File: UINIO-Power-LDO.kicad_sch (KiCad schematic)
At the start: 24 parts, among them J1 Conn_01x03_Pin, U1 ME6211C33M5G-N, U2 XC6206PxxxMR, U3 SGM2019-3.3YN5G, U4 AMS1117

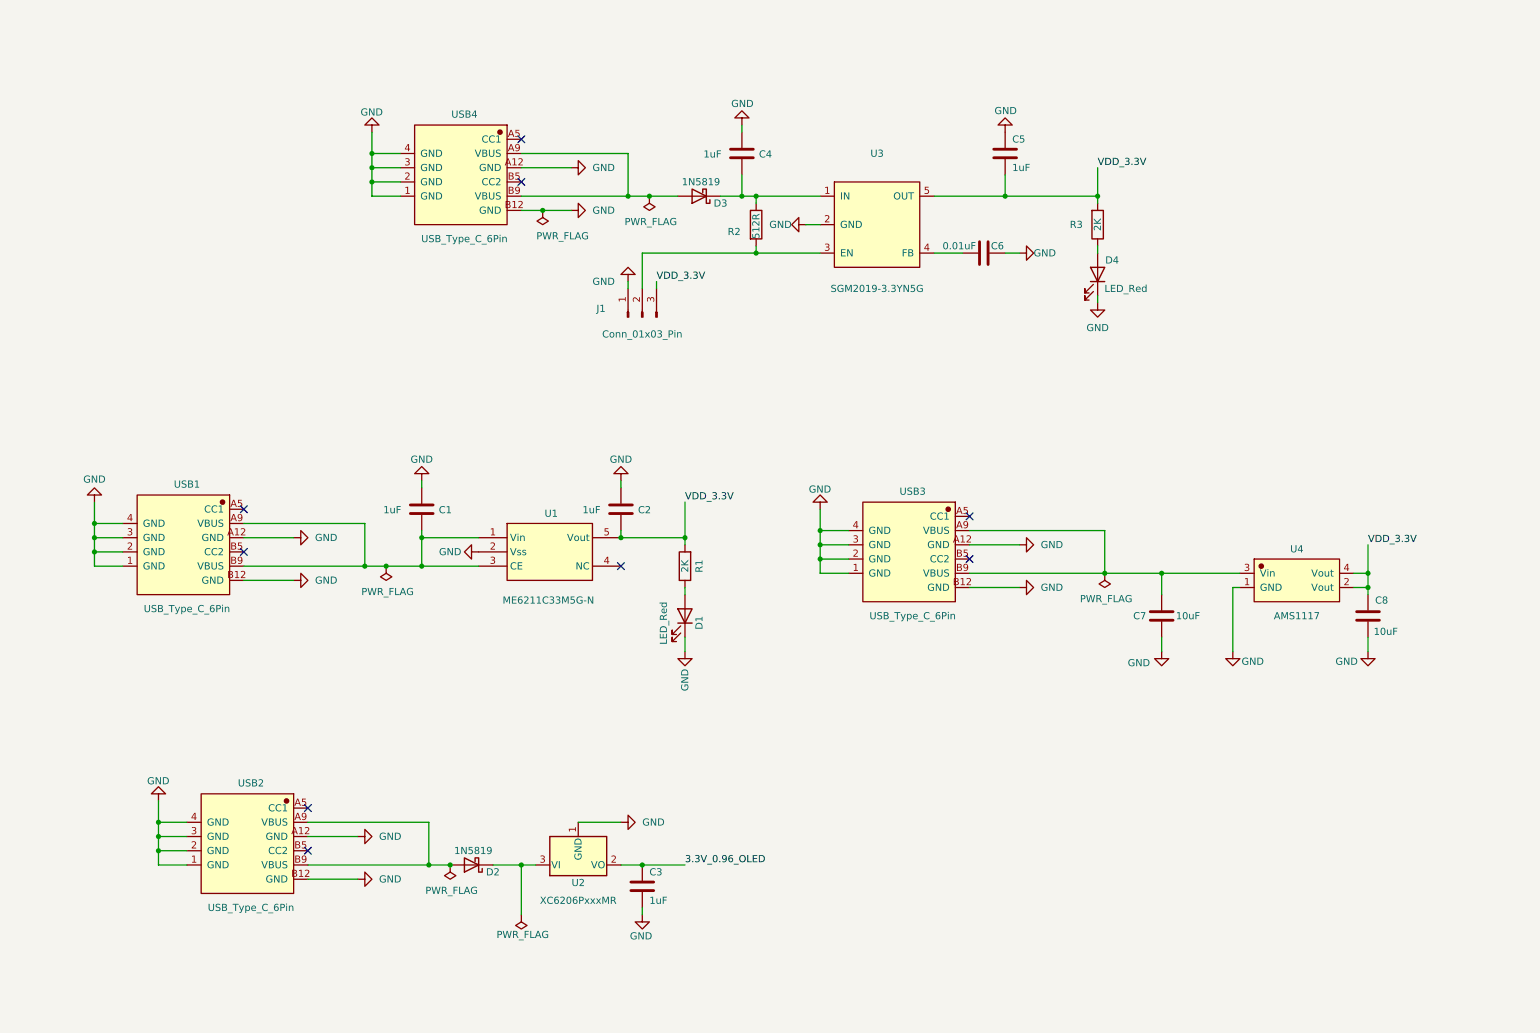
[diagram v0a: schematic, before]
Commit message: Initialization project.
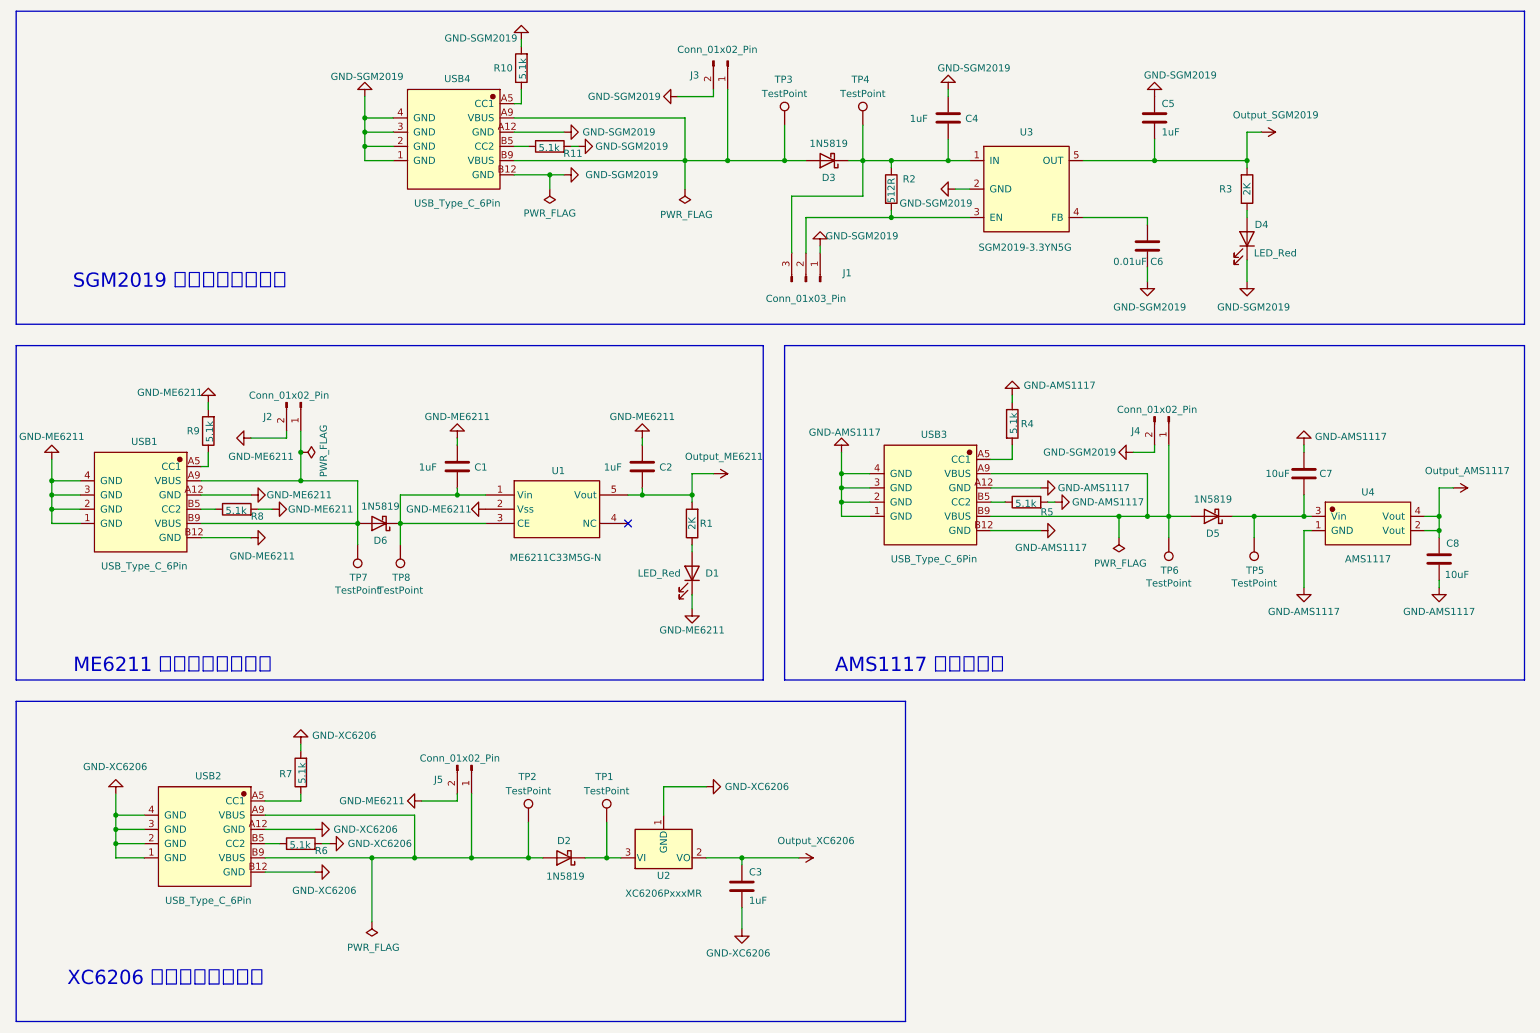
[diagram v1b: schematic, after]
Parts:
- added D5, D6: 1N5819, Diode_THT:D_DO-41_SOD81_P10.16mm_Horizontal, symbol Diode:1N5819
- added J2, J3, J4, J5: Conn_01x02_Pin, Connector_PinHeader_2.54mm:PinHeader_1x02_P2.54mm_Vertical, symbol Connector:Conn_01x02_Pin
- added R10, R11, R4, R5, R6, R7, R8, R9: 5.1k, Resistor_SMD:R_0603_1608Metric, symbol Device:R
- added TP1, TP2, TP3, TP4, TP5, TP6, TP7, TP8: TestPoint, TestPoint:TestPoint_Pad_1.5x1.5mm, symbol Connector:TestPoint
- C1, C2, C3, C7, C8: footprint Capacitor_SMD:C_0402_1005Metric -> Capacitor_SMD:C_0603_1608Metric
- J1: footprint (none) -> Connector_PinHeader_2.54mm:PinHeader_1x03_P2.54mm_Vertical
- R1: footprint Resistor_SMD:R_0402_1005Metric -> Resistor_SMD:R_0603_1608Metric
- U4: footprint kicad_lceda:SOT-223-3_L6.6-W3.5-P2.30-LS7.0-BL -> Uinio:SOT-223-3_L6.6-W3.5-P2.30-LS7.0-BL
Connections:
- net at USB2.A5 (CC1): now also R7.1
- net at D2.2 (A), USB2.A9 (VBUS), USB2.B9 (VBUS): now also J5.1 (Pin_1), TP2.1
- net at USB2.B5 (CC2): now also R6.1
- net at USB1.A5 (CC1): now also R9.1
- net at C1.2, U1.1 (Vin), U1.3 (CE): now also D6.1 (K), TP8.1; no longer USB1.A9 (VBUS), USB1.B9 (VBUS)
- net at USB1.B5 (CC2): now also R8.1
- net at C4.2, D3.1 (K), R2.1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: now also J1.3 (Pin_3), TP4.1
- net at USB4.A5 (CC1): now also R10.1
- net at D3.2 (A), USB4.A9 (VBUS), USB4.B9 (VBUS): now also J3.1 (Pin_1), TP3.1
- net at USB4.B5 (CC2): now also R11.1
- net at USB3.A9 (VBUS), USB3.B9 (VBUS): now also D5.2 (A), J4.1 (Pin_1), TP6.1; no longer C7.1, U4.3 (Vin)
- net at D2.1 (K), U2.3 (VI): now also TP1.1
- net at USB3.A5 (CC1): now also R4.2
- net at USB3.B5 (CC2): now also R5.1
- net 3.3V_0.96_OLED renamed Output_XC6206
- removed net GND: C1.1, C2.1, C3.2, C4.1, C5.1, C6.1, C7.2, C8.2, D1.1 (K), D4.1 (K), J1.1 (Pin_1), U1.2 (Vss), U2.1 (GND), U3.2 (GND), U4.1 (GND), USB1.1 (GND), USB1.2 (GND), USB1.3 (GND), USB1.4 (GND), USB1.A12 (GND), USB1.B12 (GND), USB2.1 (GND), USB2.2 (GND), USB2.3 (GND), USB2.4 (GND), USB2.A12 (GND), USB2.B12 (GND), USB3.1 (GND), USB3.2 (GND), USB3.3 (GND), USB3.4 (GND), USB3.A12 (GND), USB3.B12 (GND), USB4.1 (GND), USB4.2 (GND), USB4.3 (GND), USB4.4 (GND), USB4.A12 (GND), USB4.B12 (GND)
- removed net VDD_3.3V: C2.2, C5.2, C8.1, J1.3 (Pin_3), R1.2, R3.2, U1.5 (Vout), U3.5 (OUT), U4.2 (Vout), U4.4 (Vout)
- new net: D6.2 (A), J2.1 (Pin_1), TP7.1, USB1.A9 (VBUS), USB1.B9 (VBUS)
- new net: C7.1, D5.1 (K), TP5.1, U4.3 (Vin)
- new net GND-AMS1117: C7.2, C8.2, R4.1, R5.2, U4.1 (GND), USB3.1 (GND), USB3.2 (GND), USB3.3 (GND), USB3.4 (GND), USB3.A12 (GND), USB3.B12 (GND)
- new net GND-ME6211: C1.1, C2.1, D1.1 (K), J2.2 (Pin_2), J5.2 (Pin_2), R8.2, R9.2, U1.2 (Vss), USB1.1 (GND), USB1.2 (GND), USB1.3 (GND), USB1.4 (GND), USB1.A12 (GND), USB1.B12 (GND)
- new net GND-SGM2019: C4.1, C5.1, C6.1, D4.1 (K), J1.1 (Pin_1), J3.2 (Pin_2), J4.2 (Pin_2), R10.2, R11.2, U3.2 (GND), USB4.1 (GND), USB4.2 (GND), USB4.3 (GND), USB4.4 (GND), USB4.A12 (GND), USB4.B12 (GND)
- new net GND-XC6206: C3.2, R6.2, R7.2, U2.1 (GND), USB2.1 (GND), USB2.2 (GND), USB2.3 (GND), USB2.4 (GND), USB2.A12 (GND), USB2.B12 (GND)
- new net Output_AMS1117: C8.1, U4.2 (Vout), U4.4 (Vout)
- new net Output_ME6211: C2.2, R1.2, U1.5 (Vout)
- new net Output_SGM2019: C5.2, R3.2, U3.5 (OUT)
- no-connect marks 9 -> 1
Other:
- note added: "AMS1117 线性稳压器"
- note added: "ME6211 低压差线性稳压器"
- note added: "SGM2019 低压差线性稳压器"
- note added: "XC6206 低压差线性稳压器"
- moved on the sheet: C1, C2, C3, C4, C5, C6, C7, C8, D1, D2, D3, D4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
